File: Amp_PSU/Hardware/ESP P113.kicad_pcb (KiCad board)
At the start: 2 copper layers, 100.3 x 72.4 mm, 61 parts, among them J1 L_In, J2 R_In, J3 L_Out, J4 R_Out, J5 AC_In, Q1 MJE15032, Q2 MJE15033, Q3 MJE15032, Q4 MJE15033, U1 LM4562

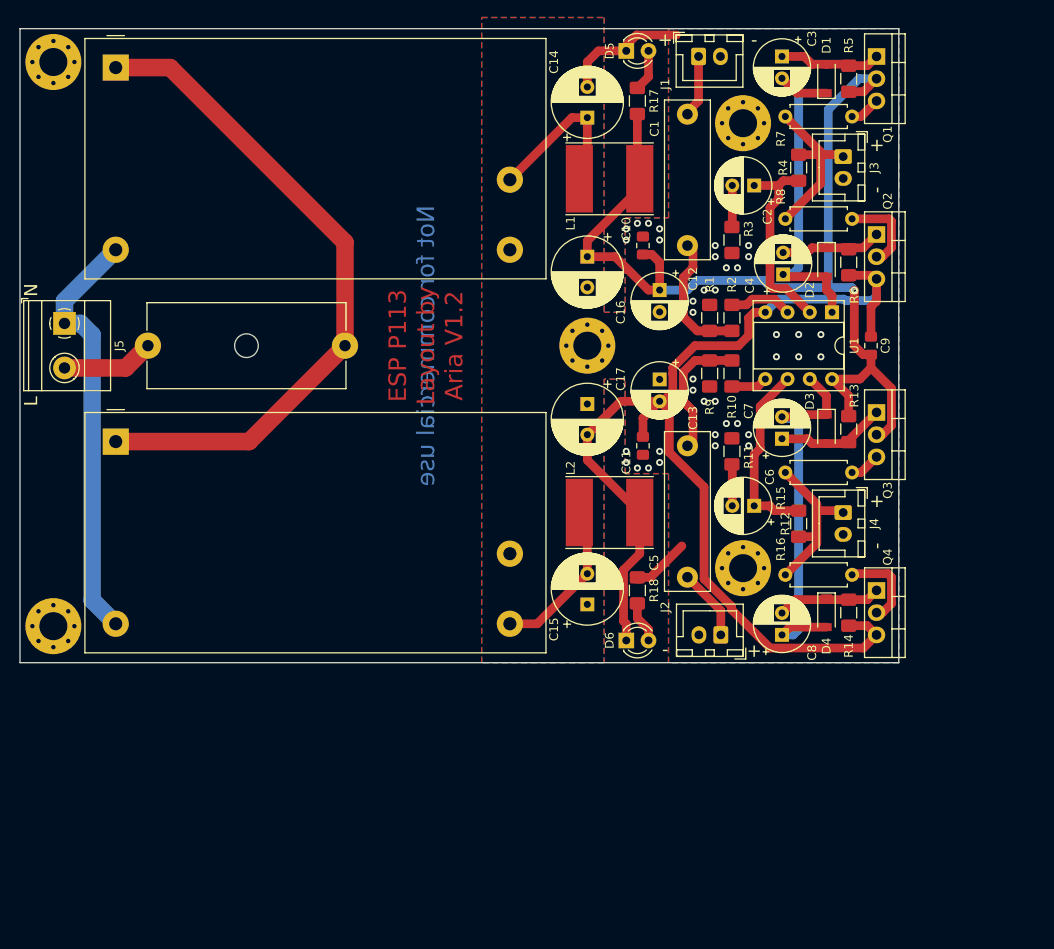
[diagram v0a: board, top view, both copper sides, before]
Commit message: Updated to V2.0.
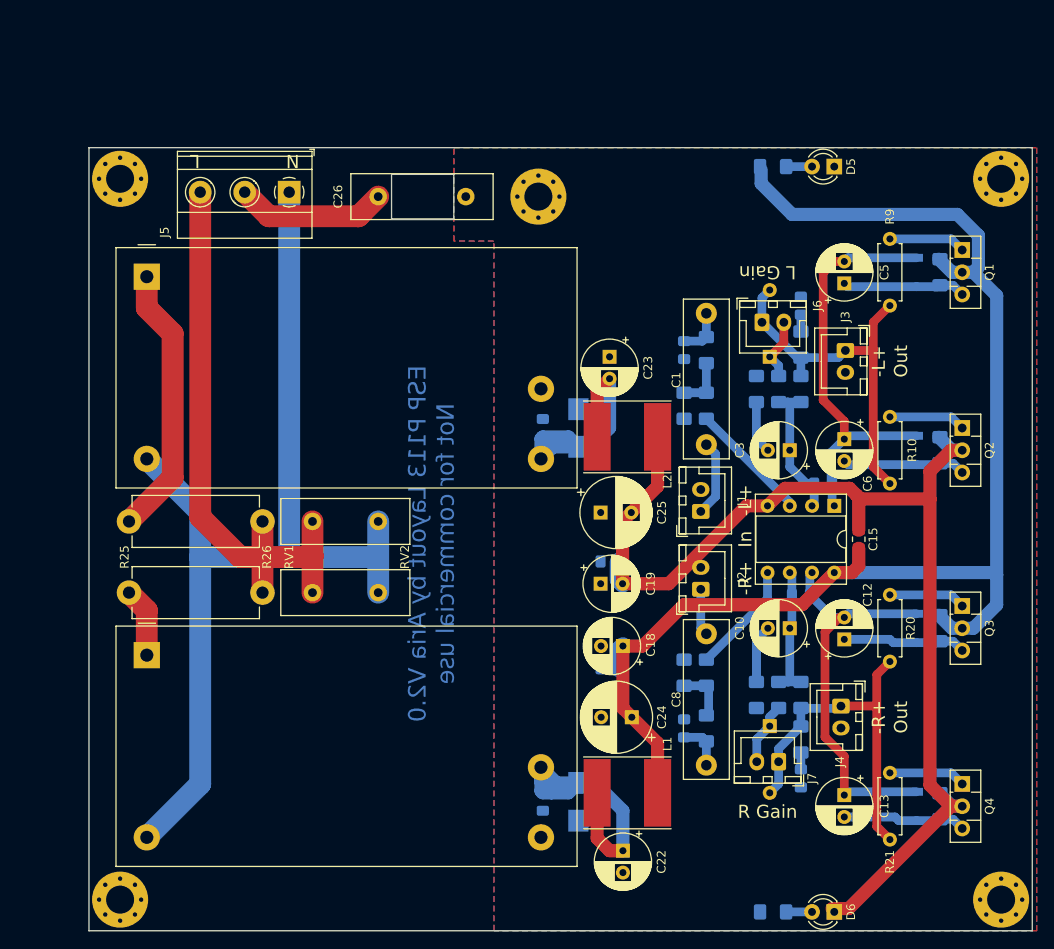
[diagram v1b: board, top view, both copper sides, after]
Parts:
- removed F1: Fuse_Small, Fuse:Fuseholder_Cylinder-5x20mm_Schurter_0031_8201_Horizontal_Open
- added C18: 100u, Capacitor_THT:CP_Radial_D6.3mm_P2.50mm, F.Cu at (128.5, 96.5)
- added C19: 100u, Capacitor_THT:CP_Radial_D6.3mm_P2.50mm, F.Cu at (126.0, 89.4)
- added C20: 1u, Capacitor_SMD:C_0805_2012Metric_Pad1.15x1.40mm_HandSolder, B.Cu at (119.4, 114.3)
- added C21: 1u, Capacitor_SMD:C_0805_2012Metric_Pad1.15x1.40mm_HandSolder, B.Cu at (119.4, 71.6)
- added C22: 10u, Capacitor_THT:CP_Radial_D6.3mm_P2.50mm, F.Cu at (128.5, 119.9)
- added C23: 10u, Capacitor_THT:CP_Radial_D6.3mm_P2.50mm, F.Cu at (127.0, 63.5)
- added C24: 220u, Capacitor_THT:CP_Radial_D8.0mm_P3.50mm, F.Cu at (129.5, 104.6)
- added C25: 220u, Capacitor_THT:CP_Radial_D8.0mm_P3.50mm, F.Cu at (126.0, 81.3)
- added C26: 10nF, Capacitor_THT:C_Disc_D16.0mm_W5.0mm_P10.00mm, F.Cu at (100.6, 45.2)
- added D7: TVS, Diode_SMD:D_SMB, B.Cu at (123.4, 114.3)
- added D8: TVS, Diode_SMD:D_SMB, B.Cu at (123.4, 71.6)
- added J6: Gain_L_Ex, Connector_JST:JST_XH_B2B-XH-A_1x02_P2.50mm_Vertical, F.Cu at (144.4, 59.6)
- added J7: Gain_R_Ex, Connector_JST:JST_XH_B2B-XH-A_1x02_P2.50mm_Vertical, F.Cu at (146.3, 109.7)
- added R19: 6k8, Resistor_SMD:R_1206_3216Metric_Pad1.42x1.75mm_HandSolder, B.Cu at (164.7, 114.8)
- added R20: 10, Resistor_THT:R_Axial_DIN0207_L6.3mm_D2.5mm_P7.62mm_Horizontal, F.Cu at (159.0, 90.7)
- added R21: 10, Resistor_THT:R_Axial_DIN0207_L6.3mm_D2.5mm_P7.62mm_Horizontal, F.Cu at (159.0, 118.6)
- added R22: 10, Resistor_SMD:R_1206_3216Metric_Pad1.42x1.75mm_HandSolder, B.Cu at (148.8, 107.2)
- added R23: 1k, Resistor_SMD:R_1206_3216Metric_Pad1.42x1.75mm_HandSolder, B.Cu at (145.7, 41.8)
- added R24: 1k, Resistor_SMD:R_1206_3216Metric_Pad1.42x1.75mm_HandSolder, B.Cu at (145.7, 126.9)
- added R25: 3, Resistor_THT:R_Axial_DIN0614_L14.3mm_D5.7mm_P15.24mm_Horizontal, F.Cu at (72.1, 90.4)
- added R26: 3, Resistor_THT:R_Axial_DIN0614_L14.3mm_D5.7mm_P15.24mm_Horizontal, F.Cu at (72.1, 82.3)
- added RV1: MOV, Capacitor_THT:C_Disc_D14.5mm_W5.0mm_P7.50mm, F.Cu at (93.1, 90.4)
- added RV2: MOV, Capacitor_THT:C_Disc_D14.5mm_W5.0mm_P7.50mm, F.Cu at (93.1, 82.3)
- added SW1: Gain_L, Button_Switch_THT:SW_DIP_SPSTx01_Slide_6.7x4.1mm_W7.62mm_P2.54mm_LowProfile, B.Cu at (145.3, 63.5)
- added SW2: Gain_R, Button_Switch_THT:SW_DIP_SPSTx01_Slide_6.7x4.1mm_W7.62mm_P2.54mm_LowProfile, B.Cu at (145.3, 105.7)
- C10: value 100n -> 100u; footprint Capacitor_SMD:C_0805_2012Metric_Pad1.15x1.40mm_HandSolder -> Capacitor_THT:CP_Radial_D6.3mm_P2.50mm
- C11: value 100n -> 22pF; moved to B.Cu
- C14, C16, C17: value 220u -> 100n; footprint Capacitor_THT:CP_Radial_D8.0mm_P3.50mm -> Capacitor_SMD:C_0805_2012Metric_Pad1.15x1.40mm_HandSolder; moved to B.Cu
- C15: value 220u -> 100n; footprint Capacitor_THT:CP_Radial_D8.0mm_P3.50mm -> Capacitor_SMD:C_0805_2012Metric_Pad1.15x1.40mm_HandSolder
- C2: value 100u -> 220p; footprint Capacitor_THT:CP_Radial_D6.3mm_P2.50mm -> Capacitor_SMD:C_0805_2012Metric_Pad1.15x1.40mm_HandSolder; moved to B.Cu
- C4: value 100u -> 22pF; footprint Capacitor_THT:CP_Radial_D6.3mm_P2.50mm -> Capacitor_SMD:C_0805_2012Metric_Pad1.15x1.40mm_HandSolder; moved to B.Cu
- C5: value 1u -> 100u; footprint Capacitor_THT:C_Rect_L18.0mm_W5.0mm_P15.00mm_FKS3_FKP3 -> Capacitor_THT:CP_Radial_D6.3mm_P2.50mm
- C7: value 100u -> 100n; footprint Capacitor_THT:CP_Radial_D6.3mm_P2.50mm -> Capacitor_SMD:C_0805_2012Metric_Pad1.15x1.40mm_HandSolder; moved to B.Cu
- C8: value 100u -> 1u; footprint Capacitor_THT:CP_Radial_D6.3mm_P2.50mm -> Capacitor_THT:C_Rect_L18.0mm_W5.0mm_P15.00mm_FKS3_FKP3
- C9: value 100n -> 220p; moved to B.Cu
- D1, D2, D3, D4: moved to B.Cu
- H1: value Star_Ground -> MountingHole
- H5: value MountingHole -> MountingHole_Pad
- J5: footprint TerminalBlock_Phoenix:TerminalBlock_Phoenix_MKDS-1,5-2-5.08_1x02_P5.08mm_Horizontal -> TerminalBlock_Phoenix:TerminalBlock_Phoenix_MKDS-1,5-3-5.08_1x03_P5.08mm_Horizontal
- Q1, Q3: value MJE15032 -> BD139; footprint Package_TO_SOT_THT:TO-220-3_Vertical -> Package_TO_SOT_THT:TO-126-3_Vertical
- Q2, Q4: value MJE15033 -> BD140; footprint Package_TO_SOT_THT:TO-220-3_Vertical -> Package_TO_SOT_THT:TO-126-3_Vertical
- R1: value 22k -> 470; moved to B.Cu
- R10: value 1k -> 10; footprint Resistor_SMD:R_1206_3216Metric_Pad1.42x1.75mm_HandSolder -> Resistor_THT:R_Axial_DIN0207_L6.3mm_D2.5mm_P7.62mm_Horizontal
- R11: value 1k -> 10; moved to B.Cu
- R12: value 3k3 -> 470; moved to B.Cu
- R13: value 6k8 -> 22k; moved to B.Cu
- R14: value 6k8 -> 470; moved to B.Cu
- R15: value 10 -> 1k; footprint Resistor_THT:R_Axial_DIN0207_L6.3mm_D2.5mm_P7.62mm_Horizontal -> Resistor_SMD:R_1206_3216Metric_Pad1.42x1.75mm_HandSolder; moved to B.Cu
- R16: value 10 -> 5k1; footprint Resistor_THT:R_Axial_DIN0207_L6.3mm_D2.5mm_P7.62mm_Horizontal -> Resistor_SMD:R_1206_3216Metric_Pad1.42x1.75mm_HandSolder; moved to B.Cu
- R17: value 1k -> 9k1; moved to B.Cu
- R18: value 1k -> 6k8; moved to B.Cu
- R2: value 1k -> 22k; moved to B.Cu
- R3: value 1k -> 470; moved to B.Cu
- R4: value 3k3 -> 1k; moved to B.Cu
- R5: value 6k8 -> 5k1; moved to B.Cu
- R6: value 6k8 -> 9k1; moved to B.Cu
- R7, R8: value 10 -> 6k8; footprint Resistor_THT:R_Axial_DIN0207_L6.3mm_D2.5mm_P7.62mm_Horizontal -> Resistor_SMD:R_1206_3216Metric_Pad1.42x1.75mm_HandSolder; moved to B.Cu
- R9: value 22k -> 10; footprint Resistor_SMD:R_1206_3216Metric_Pad1.42x1.75mm_HandSolder -> Resistor_THT:R_Axial_DIN0207_L6.3mm_D2.5mm_P7.62mm_Horizontal
- U1: value LM4562 -> OPA1642
- moved H2 112.6 mm to (171.7, 125.5), turned to 90 degrees
- moved H1 82.7 mm to (71.1, 125.5), turned to 90 degrees
- moved C14 79.3 mm to (148.8, 111.6)
- moved H3 71.4 mm to (71.1, 43.2), turned to 90 degrees
- moved R17 70.3 mm to (148.8, 102.1), turned to 270 degrees
- moved L1 70.1 mm to (129.0, 113.3)
- moved PS1 67.2 mm to (74.2, 97.6)
- moved H5 57.5 mm to (118.9, 45.2), turned to 90 degrees
- moved H4 53.3 mm to (171.7, 43.2), turned to 90 degrees
- moved J1 51.9 mm to (137.4, 81.2), turned to 90 degrees
- moved C13 51.9 mm to (153.8, 113.5)
- moved C9 48.6 mm to (135.5, 105.9)
- moved C16 47.1 mm to (127.0, 99.1), turned to 0 degrees
- moved C10 46.8 mm to (147.6, 94.5), turned to 180 degrees
- moved C12 45.1 mm to (153.8, 95.8), turned to 90 degrees
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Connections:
- C10 pad 1: Earth -> Net-(C10-Pad1)
- C10 pad 2: +15 -> Net-(C10-Pad2)
- C11 pad 1: -15 -> Net-(C11-Pad1)
- C11 pad 2: Earth -> Net-(C10-Pad1)
- C12 pad 1: +15 -> Net-(C12-Pad1)
- C12 pad 2: Earth -> Net-(C11-Pad1)
- C13 pad 1: Earth -> Net-(C11-Pad1)
- C13 pad 2: -15 -> Net-(C13-Pad2)
- C14 pad 1: Net-(C14-Pad1) -> GND
- C14 pad 2: Earth -> Net-(C14-Pad2)
- C15 pad 1: Earth -> -15
- C15 pad 2: Net-(C15-Pad2) -> +15
- C16 pad 1: +15 -> GND
- C16 pad 2: Earth -> +15
- C17 pad 1: Earth -> -15
- C17 pad 2: -15 -> GND
- C2 pad 1: Net-(C2-Pad1) -> GND
- C2 pad 2: Net-(C2-Pad2) -> Net-(C1-Pad1)
- C4 pad 1: Net-(C3-Pad2) -> Net-(C4-Pad1)
- C4 pad 2: Net-(C4-Pad2) -> Net-(C3-Pad1)
- C5 pad 2: R_In -> Net-(C4-Pad1)
- C6 pad 1: Net-(C6-Pad1) -> Net-(C4-Pad1)
- C7 pad 1: Net-(C7-Pad1) -> GND
- C8 pad 1: Net-(C7-Pad2) -> Net-(C8-Pad1)
- C8 pad 2: Net-(C8-Pad2) -> R_In
- C9 pad 1: -15 -> GND
- C9 pad 2: +15 -> Net-(C8-Pad1)
- D1 pad 1: Net-(C3-Pad2) -> Net-(C4-Pad1)
- D1 pad 2: Net-(C3-Pad1) -> Net-(C5-Pad1)
- D2 pad 1: Net-(C4-Pad2) -> Net-(C6-Pad2)
- D2 pad 2: Net-(C3-Pad2) -> Net-(C4-Pad1)
- D3 pad 1: Net-(C7-Pad2) -> Net-(C11-Pad1)
- D3 pad 2: Net-(C7-Pad1) -> Net-(C12-Pad1)
- D4 pad 1: Net-(C8-Pad2) -> Net-(C13-Pad2)
- D4 pad 2: Net-(C7-Pad2) -> Net-(C11-Pad1)
- D5 pad 1: Earth -> GND
- H1 pad 1: Earth -> (no net)
- H5 pad 1: (no net) -> GND
- J1 pad 2: Earth -> GND
- J2 pad 2: Earth -> GND
- J3 pad 2: Earth -> GND
- J4 pad 2: Earth -> GND
- J5 pad 2: Net-(F1-Pad1) -> GNDREF
- L1 pad 1: Net-(C14-Pad1) -> Net-(C20-Pad1)
- L2 pad 1: Net-(C15-Pad2) -> Net-(C21-Pad2)
- PS1 pad 1: Net-(F1-Pad2) -> Net-(PS1-Pad1)
- PS1 pad 3: Earth -> GND
- PS1 pad 4: Net-(C14-Pad1) -> Net-(C20-Pad1)
- PS2 pad 1: Net-(F1-Pad2) -> Net-(PS2-Pad1)
- PS2 pad 3: Net-(C15-Pad2) -> Net-(C21-Pad2)
- PS2 pad 4: Earth -> GND
- Q1 pad 1: Net-(C3-Pad1) -> Net-(Q1-Pad1)
- Q1 pad 3: Net-(Q1-Pad3) -> Net-(C5-Pad1)
- Q2 pad 1: Net-(C4-Pad2) -> Net-(Q2-Pad1)
- Q2 pad 2: Net-(Q2-Pad2) -> -15
- Q2 pad 3: -15 -> Net-(C6-Pad2)
- Q3 pad 1: Net-(C7-Pad1) -> Net-(Q3-Pad1)
- Q3 pad 3: Net-(Q3-Pad3) -> Net-(C12-Pad1)
- Q4 pad 1: Net-(C8-Pad2) -> Net-(Q4-Pad1)
- Q4 pad 2: Net-(Q4-Pad2) -> -15
- Q4 pad 3: -15 -> Net-(C13-Pad2)
- R1 pad 1: Net-(C1-Pad1) -> Net-(R1-Pad1)
- R1 pad 2: Earth -> Net-(C1-Pad1)
- R10 pad 1: Net-(R10-Pad1) -> L_Out
- R10 pad 2: Net-(C5-Pad1) -> Net-(Q2-Pad1)
- R11 pad 1: Net-(C6-Pad2) -> Net-(C7-Pad2)
- R11 pad 2: Earth -> L_Out
- R12 pad 1: Net-(C6-Pad1) -> Net-(R12-Pad1)
- R12 pad 2: R_Out -> Net-(C8-Pad1)
- R13 pad 1: +15 -> Net-(R12-Pad1)
- R13 pad 2: Net-(C7-Pad1) -> GND
- R14 pad 1: Net-(C8-Pad2) -> Net-(R14-Pad1)
- R14 pad 2: -15 -> Net-(R12-Pad1)
- R15 pad 1: Net-(Q3-Pad3) -> Net-(C10-Pad2)
- R15 pad 2: R_Out -> GND
- R16 pad 1: R_Out -> Net-(C10-Pad1)
- R16 pad 2: Net-(Q4-Pad2) -> Net-(J7-Pad2)
- R17 pad 1: +15 -> Net-(C10-Pad1)
- R17 pad 2: Net-(D5-Pad2) -> R_Out
- R18 pad 1: Earth -> +15
- R18 pad 2: Net-(D6-Pad2) -> Net-(C12-Pad1)
- R2 pad 1: Net-(R2-Pad1) -> Net-(R1-Pad1)
- R2 pad 2: Net-(C1-Pad1) -> GND
- R3 pad 1: Net-(C2-Pad2) -> Net-(R3-Pad1)
- R3 pad 2: Earth -> Net-(R1-Pad1)
- R4 pad 1: Net-(C2-Pad1) -> Net-(C3-Pad2)
- R4 pad 2: L_Out -> GND
- R5 pad 1: +15 -> Net-(C3-Pad1)
- R5 pad 2: Net-(C3-Pad1) -> Net-(J6-Pad2)
- R6 pad 1: Net-(C4-Pad2) -> Net-(C3-Pad1)
- R6 pad 2: -15 -> L_Out
- R7 pad 1: Net-(Q1-Pad3) -> +15
- R7 pad 2: L_Out -> Net-(C5-Pad1)
- R8 pad 1: L_Out -> Net-(C6-Pad2)
- R8 pad 2: Net-(Q2-Pad2) -> -15
- R9 pad 1: Net-(C5-Pad1) -> Net-(Q1-Pad1)
- R9 pad 2: Earth -> L_Out
- U1 pad 1: Net-(C3-Pad2) -> Net-(C4-Pad1)
- U1 pad 2: Net-(C2-Pad1) -> Net-(C3-Pad1)
- U1 pad 3: Net-(R2-Pad1) -> Net-(R3-Pad1)
- U1 pad 5: Net-(R10-Pad1) -> Net-(R14-Pad1)
- U1 pad 6: Net-(C6-Pad1) -> Net-(C10-Pad1)
- U1 pad 7: Net-(C7-Pad2) -> Net-(C11-Pad1)
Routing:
- net Net-(J5-Pad1): track 48.6 -> 126.5 mm
- net Net-(F1-Pad2): track 76.9 -> 0.00 mm
- net Net-(J5-Pad3): track 0.00 -> 76.2 mm
- net Net-(C4-Pad1): track 0.00 -> 48.2 mm
- net Net-(C11-Pad1): track 0.00 -> 46.9 mm
- net Net-(C7-Pad2): track 43.2 -> 1.93 mm
- net +15: track 117.6 -> 157.7 mm, vias 1 -> 0
- net Net-(C20-Pad1): track 0.00 -> 35.6 mm
- net Net-(C3-Pad2): track 39.9 -> 6.04 mm
- net Net-(PS2-Pad1): track 0.00 -> 31.2 mm
- net Net-(C21-Pad2): track 0.00 -> 29.3 mm
- net L_Out: track 20.2 -> 42.8 mm
- net Net-(C2-Pad1): track 22.5 -> 0.00 mm
- net R_Out: track 19.9 -> 41.5 mm
- net Earth: track 21.5 -> 0.00 mm, vias 38 -> 0
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- added copper zone on B.Cu, net GND
- added copper zone on F.Cu, net GND
- removed copper zone on B.Cu, net Earth
- removed copper zone on F.Cu, net Earth
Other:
- board size 100.3 x 72.4 mm -> 107.7 x 89.4 mm
- net class AC added: clearance 0.2, trace_width 2.5, via_dia 0.8, via_drill 0.4
- net class DC added: clearance 0.2, trace_width 1.5, via_dia 0.8, via_drill 0.4
- net class Power removed
- board text added: "-L+"
- board text added: "-R+"
- board text added: "ESP P113 Layout by Aria V2.0 Not for commercial use"
- board text added: "In"
- board text added: "L Gain"
- board text added: "N L"
- board text added: "Out"
- board text added: "R Gain"
- board text removed: "+"
- board text removed: "-"
- board text removed: "ESP P113 Layout by Aria V1.2"
- board text removed: "L"
- board text removed: "N"
- board text removed: "Not for commercial use"

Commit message: Changed layout
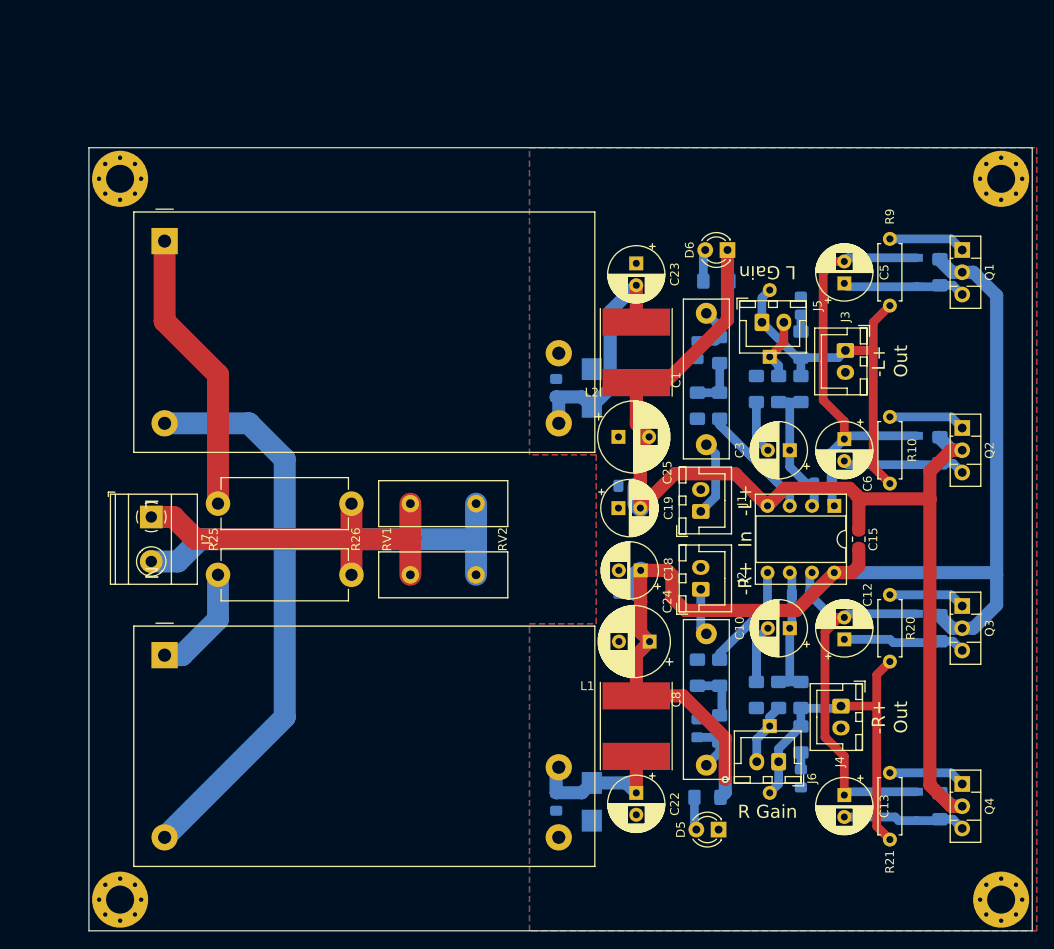
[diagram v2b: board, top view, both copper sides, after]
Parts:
- removed C26: 10nF, Capacitor_THT:C_Disc_D16.0mm_W5.0mm_P10.00mm
- removed H5: MountingHole_Pad, MountingHole:MountingHole_3.2mm_M3_Pad_Via
- removed the J5 at (90.4, 44.7)
- added J7: AC_In, TerminalBlock_Phoenix:TerminalBlock_Phoenix_MKDS-1,5-2-5.08_1x02_P5.08mm_Horizontal, F.Cu at (74.7, 81.8)
- moved D5 76.8 mm to (139.4, 117.5)
- moved D6 76.5 mm to (140.5, 51.3)
- moved R23 72.4 mm to (138.2, 113.8), turned to 180 degrees
- moved R24 72.3 mm to (139.2, 54.9), turned to 180 degrees
- moved RV1 11.4 mm to (104.3, 88.4)
- moved RV2 11.4 mm to (104.3, 80.3)
- moved C23 11.1 mm to (130.0, 52.8)
- moved R25 10.4 mm to (82.3, 88.4)
- moved R26 10.4 mm to (82.3, 80.3)
- moved L2 9.71 mm to (130.0, 63.0), turned to 270 degrees
- moved C16 8.87 mm to (129.0, 90.4)
- moved C17 8.87 mm to (129.0, 78.2)
- moved C18 8.87 mm to (130.6, 87.9)
- moved C24 8.87 mm to (131.6, 96.0)
- moved C19 8.87 mm to (128.0, 80.8)
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- renumbered J6 to J5, J7 to J6
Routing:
- net Net-(J7-Pad1): track 76.2 -> 46.9 mm
- net Net-(C20-Pad1): track 35.6 -> 17.3 mm
- net +15: track 157.7 -> 140.3 mm, vias 0 -> 1
- net GNDREF: track 17.3 -> 0.00 mm
- net Net-(J7-Pad2): track 126.5 -> 110.5 mm
- net -15: track 135.6 -> 132.8 mm
- net Net-(C21-Pad2): track 29.3 -> 27.9 mm
- net Net-(PS2-Pad1): track 31.2 -> 32.5 mm
- net Net-(D5-Pad2): track 2.96 -> 3.77 mm
- net Net-(D6-Pad2): track 2.96 -> 3.65 mm
- net Net-(C1-Pad1): track 5.45 -> 6.08 mm
- net Net-(R14-Pad1): track 12.8 -> 12.2 mm
- net Net-(R3-Pad1): track 13.9 -> 13.3 mm
- net Net-(C8-Pad1): track 5.45 -> 6.08 mm
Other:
- outline, holes or cut-outs redrawn
- board text added: "L N"
- board text removed: "N L"
